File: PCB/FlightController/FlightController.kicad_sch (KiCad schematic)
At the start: 13 parts, among them J1 SMA Connector, J2 BATT IN, J3 BATT OUT, J4 BATT Reg IC, J5 Pump, J7 HallCircuit, Q1 P_CHANNEL, U1 XIAO-nRF52840-DIP, U2 RFM95W

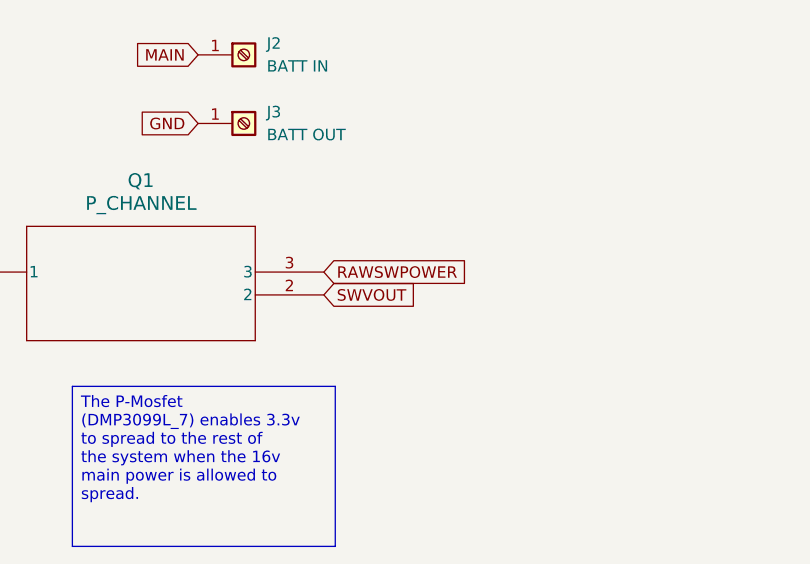
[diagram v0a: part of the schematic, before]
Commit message: All boards should be finished. ACC otw, and an earlier version of the main board otw
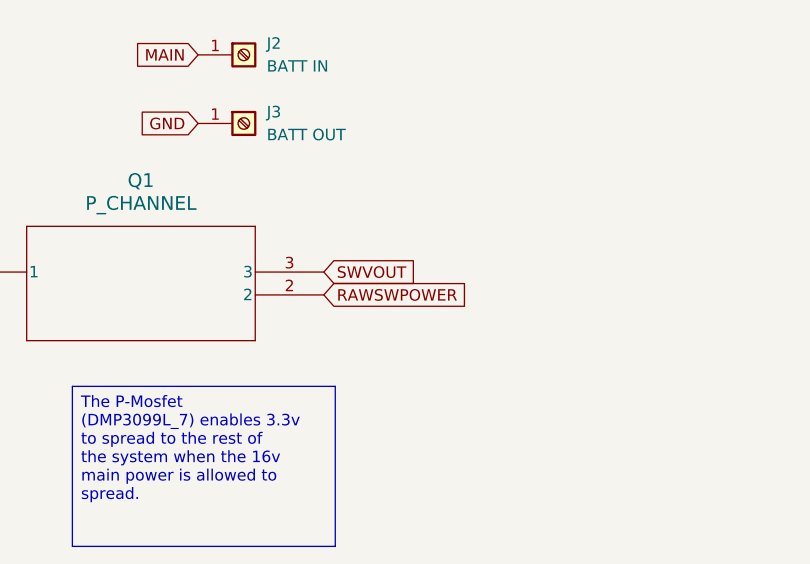
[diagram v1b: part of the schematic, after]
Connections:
- net RAWSWPOWER: now also Q1.2; no longer Q1.3
- net SWVOUT: now also Q1.3; no longer Q1.2
